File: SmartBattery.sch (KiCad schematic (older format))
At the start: 52 parts

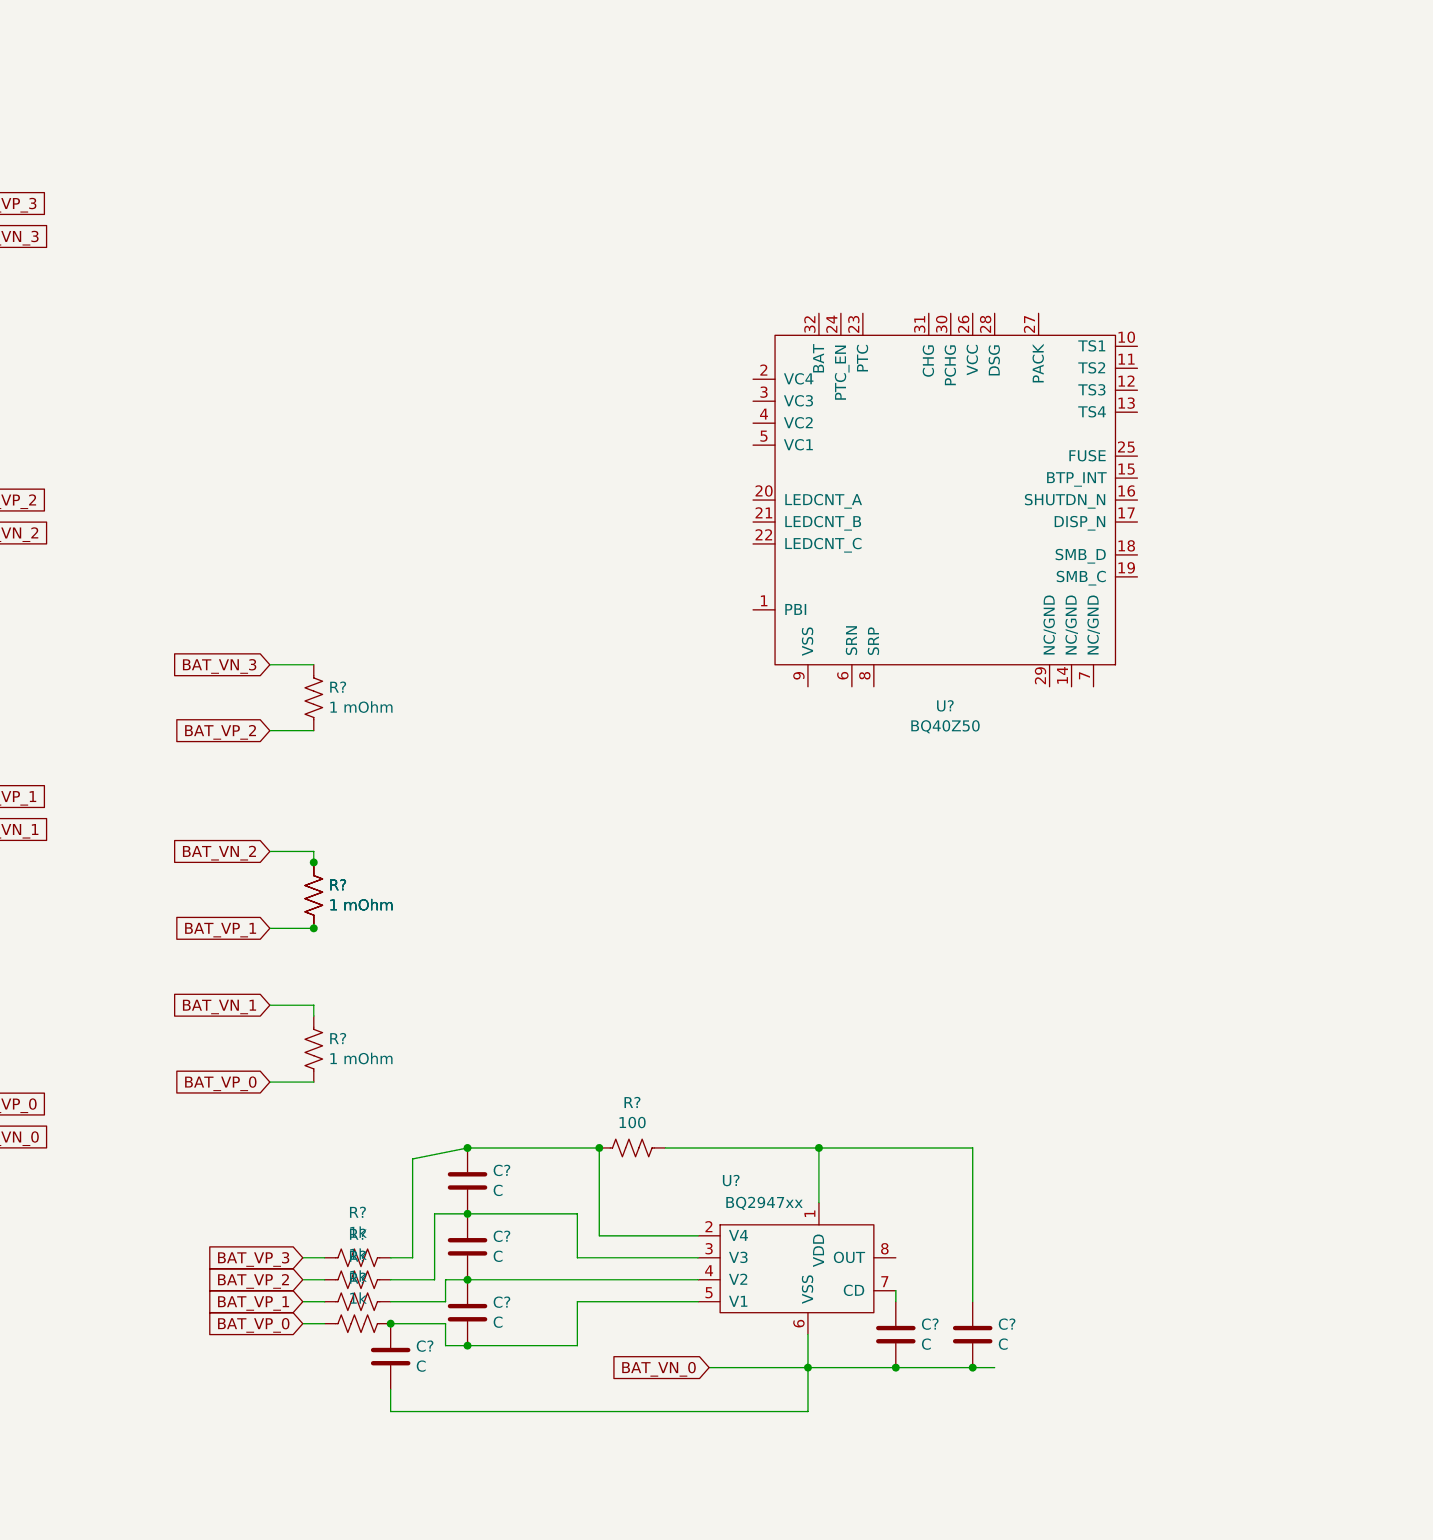
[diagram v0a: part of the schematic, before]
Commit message: added some more protection connection
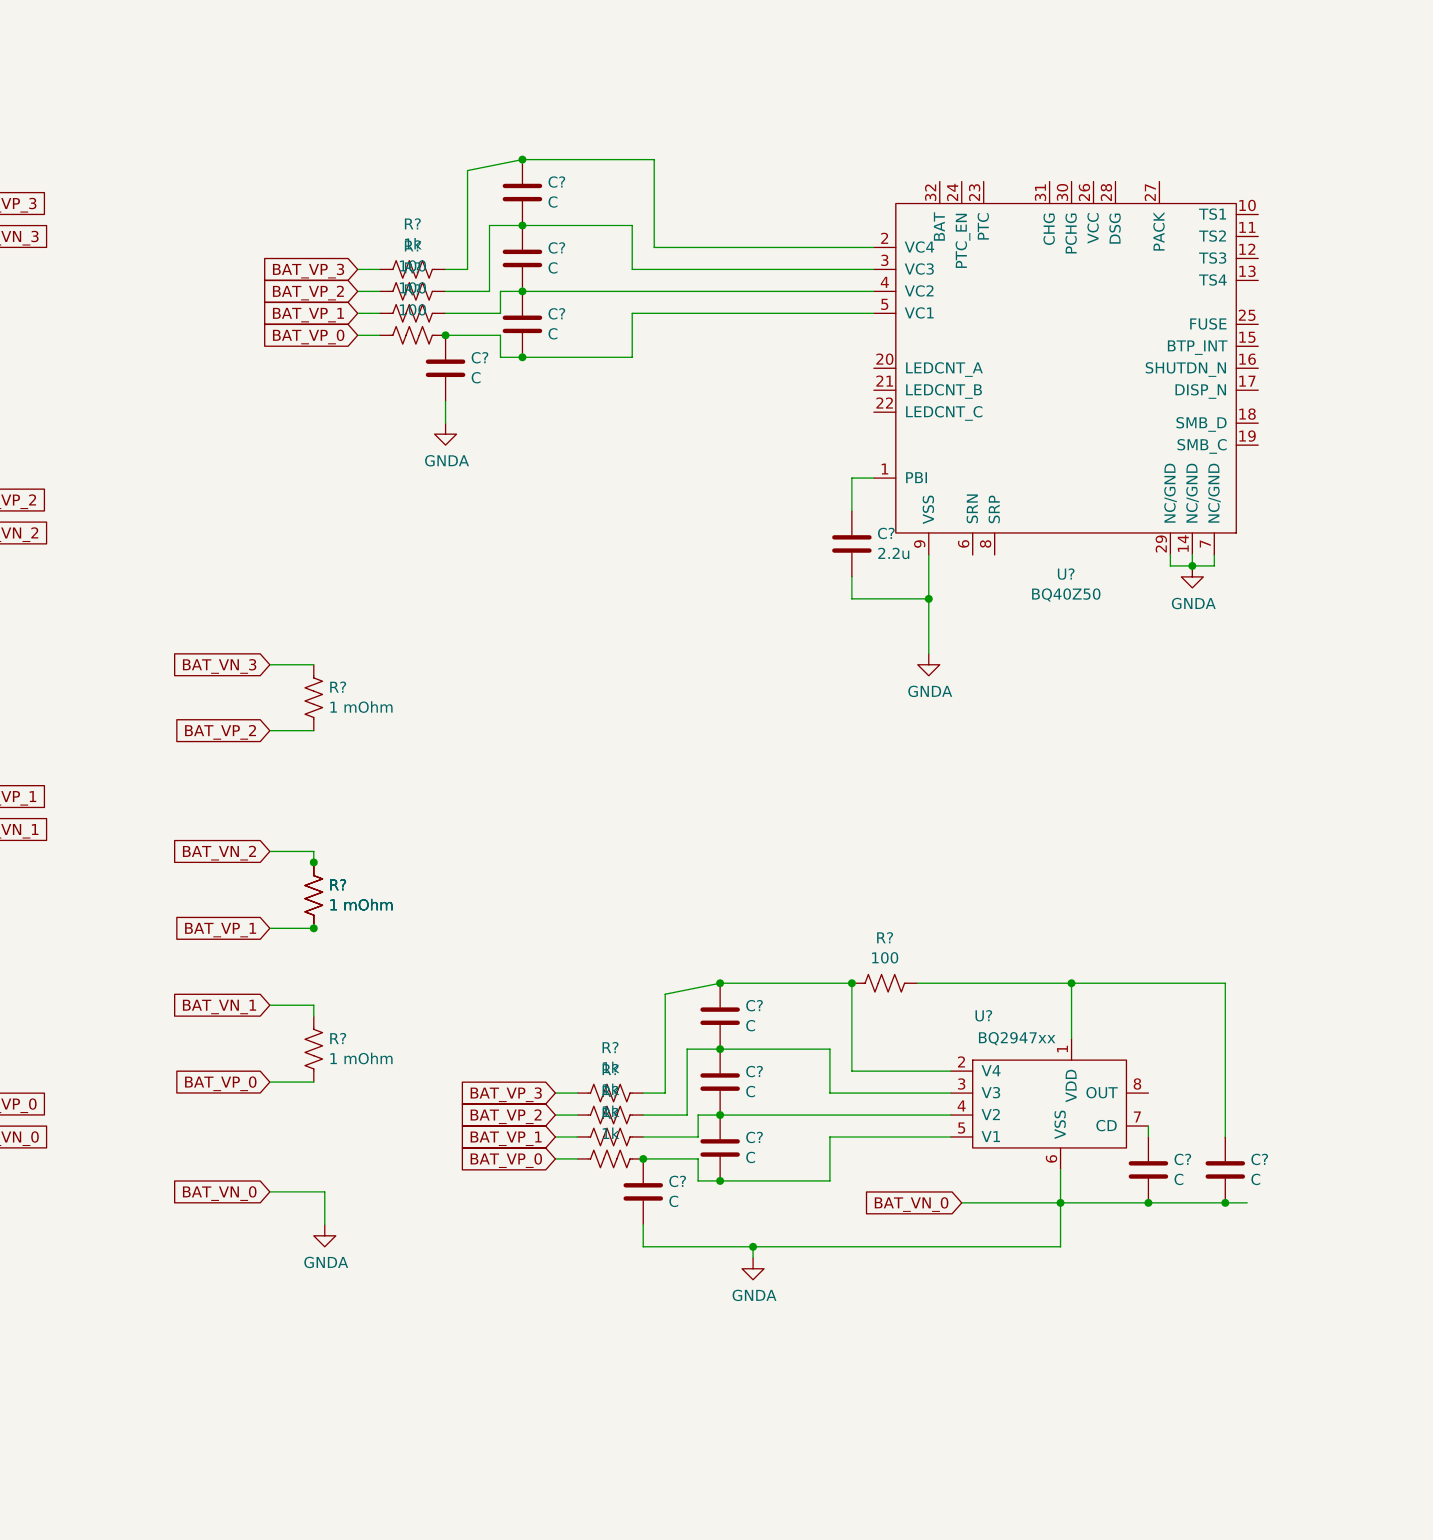
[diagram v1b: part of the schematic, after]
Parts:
- added C? (x4): C, symbol Device:C
- added C?: 2.2u, symbol Device:C
- added R? (x3): 100, 0201, symbol Device:R_US
- added R?: 1k, 0201, symbol Device:R_US
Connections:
- net BAT_VN_0 is gone; now on net GNDA: C?.2, C?.2, C?.2, J?.2 (Pin_2), J?.2 (Pin_2), TP?.1, U?.6 (VSS)
- net BAT_VP_0: now also R?.2
- net BAT_VP_1: now also R?.2
- net BAT_VP_2: now also R?.2
- net BAT_VP_3: now also R?.2
- net at U?.1 (PBI): now also C?.1
- net GNDA: now reaches U?.14 (NC/GND)
- net GNDA: now also U?.29 (NC/GND), U?.7 (NC/GND), U?.9 (VSS), C?.2, C?.2
- net at U?.2 (VC4): now also C?.1, R?.1
- net at U?.3 (VC3): now also C?.1, C?.2, R?.1
- net at U?.4 (VC2): now also C?.1, C?.2, R?.1
- net at U?.5 (VC1): now also C?.1, C?.2, R?.1
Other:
- moved on the sheet: C?, R?, U?
